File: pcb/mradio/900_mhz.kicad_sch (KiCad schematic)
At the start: 20 parts, among them J401 MM60-52B1-E1-R650, U401 74AVC4T774, U402 74AVC4T774

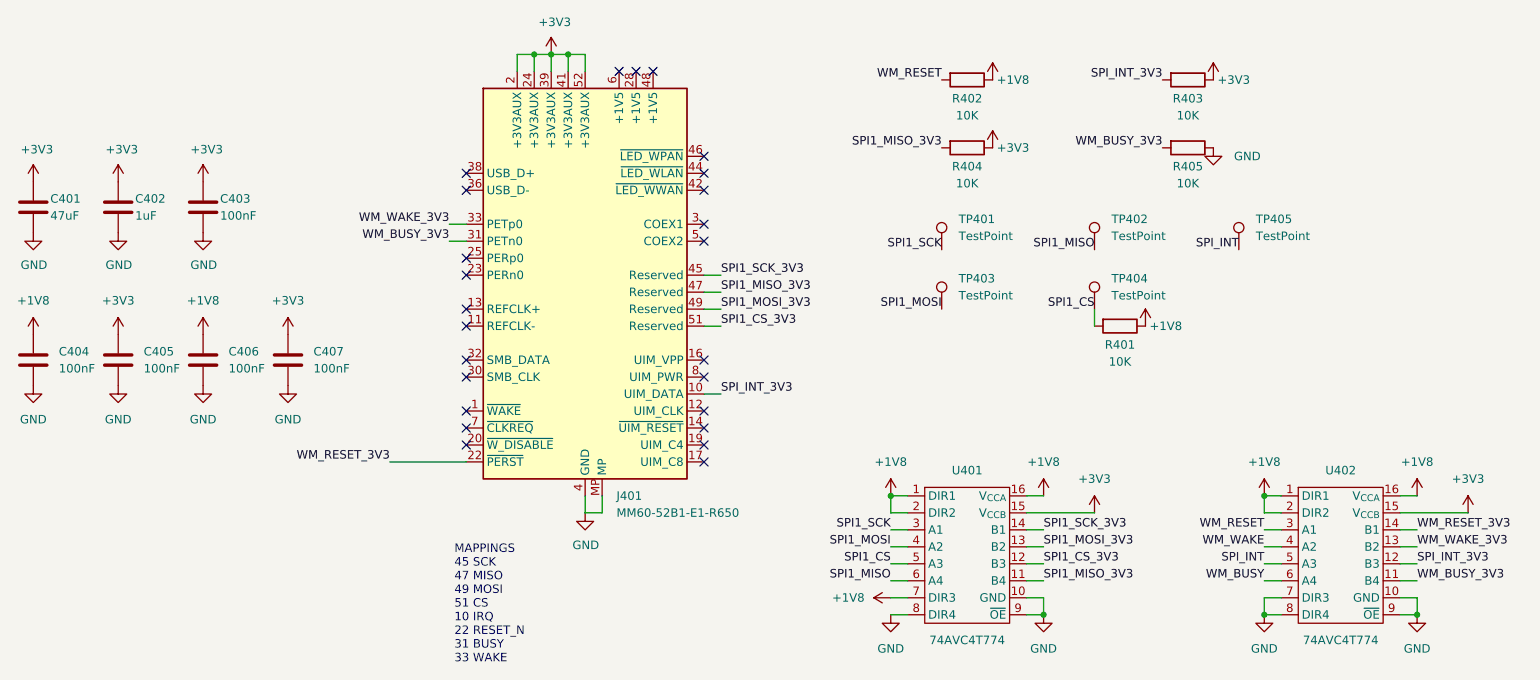
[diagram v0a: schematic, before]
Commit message: Fixed numbers
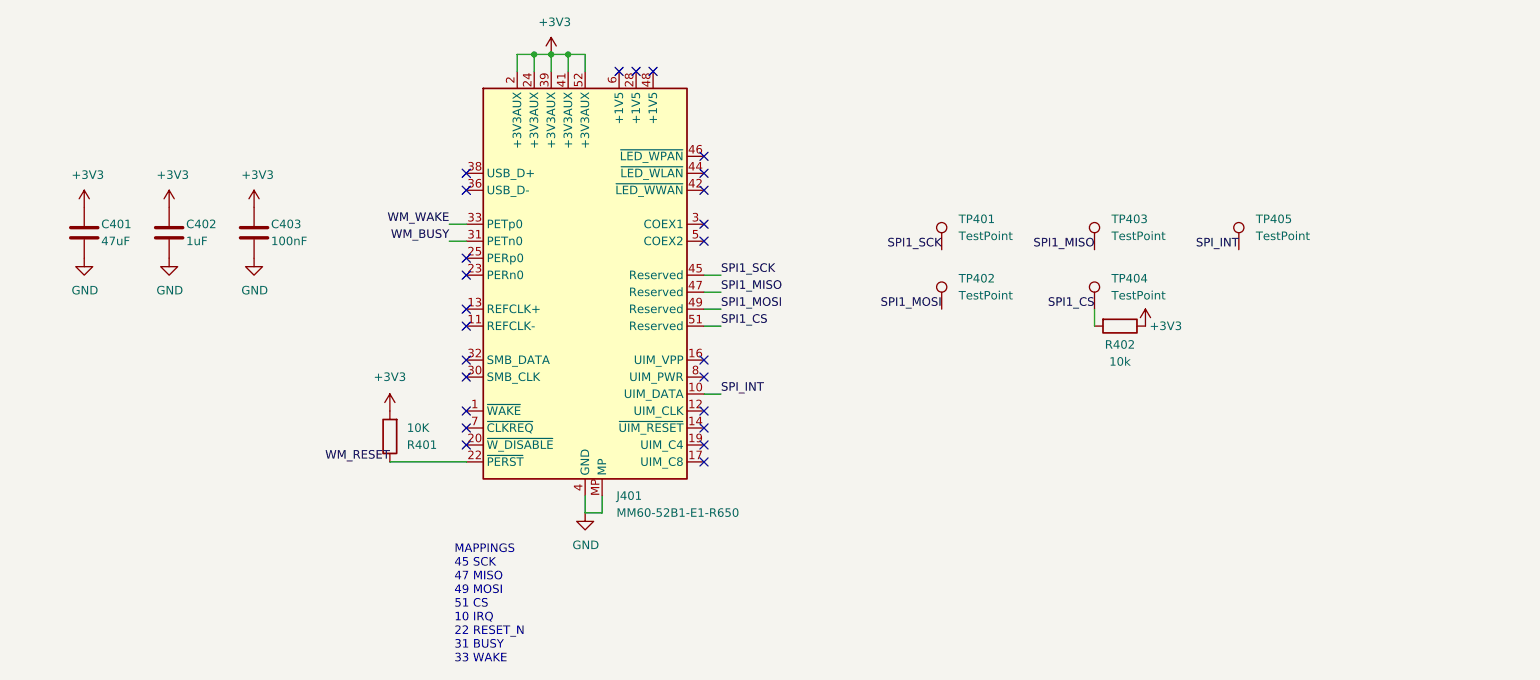
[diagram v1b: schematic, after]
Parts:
- removed C404, C405, C406, C407: 100nF, Capacitor_SMD:C_0603_1608Metric, symbol Device:C
- removed R402, R403, R404, R405: 10K, Resistor_SMD:R_0603_1608Metric, symbol Device:R
- removed U401, U402: 74AVC4T774, Package_SO:TSSOP-16_4.4x5mm_P0.65mm, symbol 74AVC4T774QPWRQ1:74AVC4T774QPWRQ1
- added R401: 10K, Resistor_SMD:R_0603_1608Metric, symbol Device:R
- R402: renamed from R401; value 10K -> 10k; footprint Resistor_SMD:R_0603_1608Metric -> (none)
- TP401, TP404, TP405: footprint TestPoint:TestPoint_Pad_D1.0mm -> (none)
- TP402: renamed from TP403; footprint TestPoint:TestPoint_Pad_D1.0mm -> (none)
- TP403: renamed from TP402; footprint TestPoint:TestPoint_Pad_D1.0mm -> (none)
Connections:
- net +1V8 is gone; now on net +3V3: R402.1
- net SPI1_CS_3V3 is gone; now on net SPI1_CS: J401.51 (Reserved)
- net SPI1_MISO_3V3 is gone; now on net SPI1_MISO: J401.47 (Reserved)
- net SPI1_MOSI_3V3 is gone; now on net SPI1_MOSI: J401.49 (Reserved)
- net SPI1_SCK_3V3 is gone; now on net SPI1_SCK: J401.45 (Reserved)
- net SPI_INT_3V3 is gone; now on net SPI_INT: J401.10 (UIM_DATA)
- net WM_BUSY_3V3 is gone; now on net WM_BUSY: J401.31 (PETn0)
- net WM_RESET_3V3 is gone; now on net WM_RESET: J401.22 (~{PERST})
- net WM_WAKE_3V3 is gone; now on net WM_WAKE: J401.33 (PETp0)
- net +3V3: now also R401.2
- net WM_RESET: now also R401.1
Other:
- moved on the sheet: C401, C402, C403

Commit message: undid overwrite
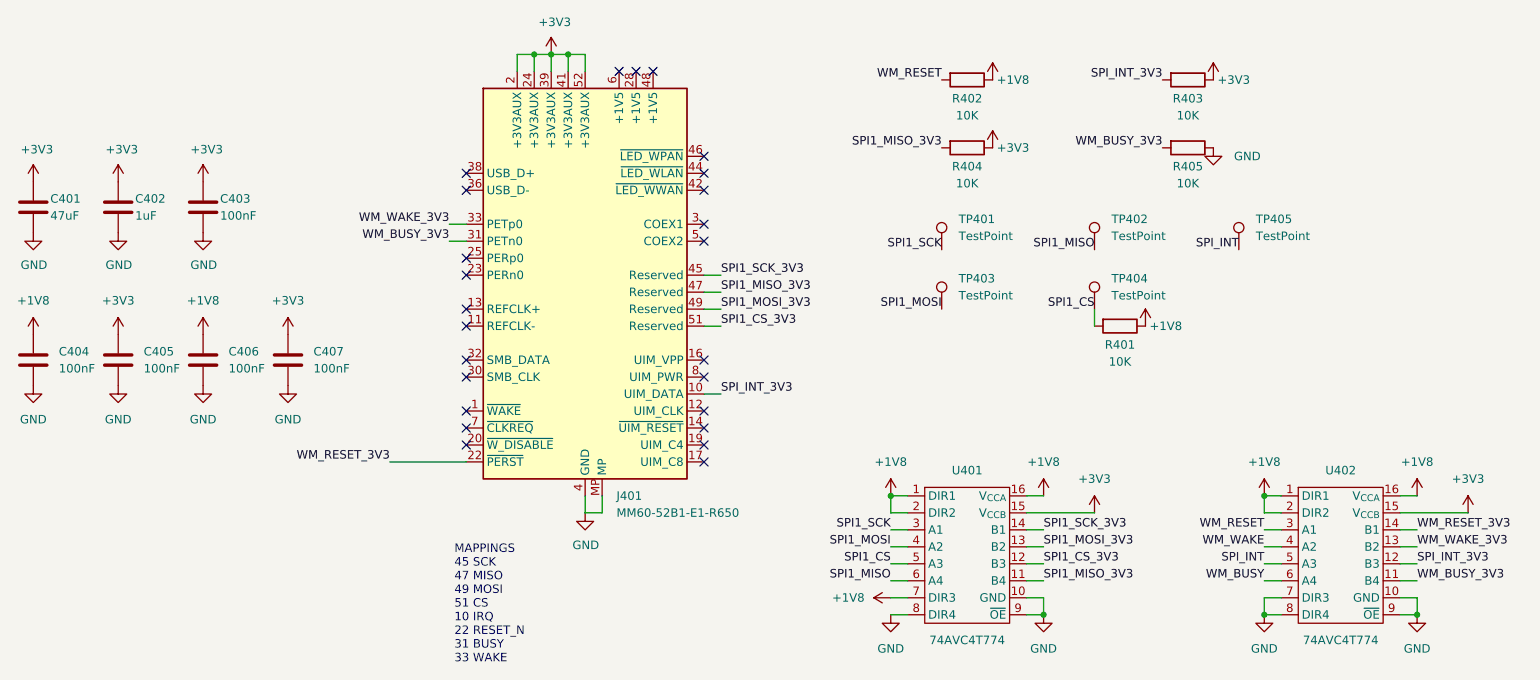
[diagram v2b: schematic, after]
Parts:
- removed R401: 10K, Resistor_SMD:R_0603_1608Metric, symbol Device:R
- added C404, C405, C406, C407: 100nF, Capacitor_SMD:C_0603_1608Metric, symbol Device:C
- added R402, R403, R404, R405: 10K, Resistor_SMD:R_0603_1608Metric, symbol Device:R
- added U401, U402: 74AVC4T774, Package_SO:TSSOP-16_4.4x5mm_P0.65mm, symbol 74AVC4T774QPWRQ1:74AVC4T774QPWRQ1
- R401: renamed from R402; value 10k -> 10K; footprint (none) -> Resistor_SMD:R_0603_1608Metric
- TP401, TP404, TP405: footprint (none) -> TestPoint:TestPoint_Pad_D1.0mm
- TP402: renamed from TP403; footprint (none) -> TestPoint:TestPoint_Pad_D1.0mm
- TP403: renamed from TP402; footprint (none) -> TestPoint:TestPoint_Pad_D1.0mm
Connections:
- net +3V3: now also C405.1, C407.1, R403.1, R404.1, U401.15 (V_{CCB}), U402.15 (V_{CCB}); no longer R401.1
- net GND: now also C404.2, C405.2, C406.2, C407.2, R405.1, U401.10 (GND), U401.8 (DIR4), U401.9 (~{OE}), U402.10 (GND), U402.7 (DIR3), U402.8 (DIR4), U402.9 (~{OE})
- net SPI1_CS: now also U401.5 (A3); no longer J401.51 (Reserved)
- net SPI1_MISO: now also U401.6 (A4); no longer J401.47 (Reserved)
- net SPI1_MOSI: now also U401.4 (A2); no longer J401.49 (Reserved)
- net SPI1_SCK: now also U401.3 (A1); no longer J401.45 (Reserved)
- net SPI_INT: now also U402.5 (A3); no longer J401.10 (UIM_DATA)
- net WM_BUSY: now also U402.6 (A4); no longer J401.31 (PETn0)
- net WM_RESET: now also R402.2, U402.3 (A1); no longer J401.22 (~{PERST})
- net WM_WAKE: now also U402.4 (A2); no longer J401.33 (PETp0)
- new net +1V8: C404.1, C406.1, R401.1, R402.1, U401.1 (DIR1), U401.16 (V_{CCA}), U401.2 (DIR2), U401.7 (DIR3), U402.1 (DIR1), U402.16 (V_{CCA}), U402.2 (DIR2)
- new net SPI1_CS_3V3: J401.51 (Reserved), U401.12 (B3)
- new net SPI1_MISO_3V3: J401.47 (Reserved), R404.2, U401.11 (B4)
- new net SPI1_MOSI_3V3: J401.49 (Reserved), U401.13 (B2)
- new net SPI1_SCK_3V3: J401.45 (Reserved), U401.14 (B1)
- new net SPI_INT_3V3: J401.10 (UIM_DATA), R403.2, U402.12 (B3)
- new net WM_BUSY_3V3: J401.31 (PETn0), R405.2, U402.11 (B4)
- new net WM_RESET_3V3: J401.22 (~{PERST}), U402.14 (B1)
- new net WM_WAKE_3V3: J401.33 (PETp0), U402.13 (B2)
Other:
- moved on the sheet: C401, C402, C403
